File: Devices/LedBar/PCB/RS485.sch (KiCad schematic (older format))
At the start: 20 parts, among them J401 RS485, U401 ISO3082DW, U402 B0505S-1W-SIP4

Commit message: Renamed libraries
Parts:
- J401: footprint AmbientLight:15EDGRC-3.5-3P -> RGBW-Bar:15EDGRC-3.5-3P
- TP401, TP402, TP403, TP404, TP405, TP406, TP407, TP408, TP409: footprint AmbientLight:TestPoint_Pad_D1.0mm -> RGBW-Bar:TestPoint_Pad_D1.0mm
- U402: footprint AmbientLight:B0505S-1W -> RGBW-Bar:B0505S-1W; symbol AmbientLight:B0505S-1W-SIP4 -> RGBW-Bar:B0505S-1W-SIP4
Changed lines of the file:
@@
 F 0 "TP406" H 7658 4468 50  0000 L CNN
 F 1 "txd" H 7658 4377 50  0000 L CNN
-F 2 "AmbientLight:TestPoint_Pad_D1.0mm" H 7800 4350 50  0001 C CNN
+F 2 "RGBW-Bar:TestPoint_Pad_D1.0mm" H 7800 4350 50  0001 C CNN
 F 3 "~" H 7800 4350 50  0001 C CNN
 	1    7600 4350
@@
 F 0 "TP407" H 7542 4676 50  0000 R CNN
 F 1 "rxd" H 7542 4767 50  0000 R CNN
-F 2 "AmbientLight:TestPoint_Pad_D1.0mm" H 7800 4650 50  0001 C CNN
+F 2 "RGBW-Bar:TestPoint_Pad_D1.0mm" H 7800 4650 50  0001 C CNN
 F 3 "~" H 7800 4650 50  0001 C CNN
 	1    7600 4650
@@
 F 0 "TP408" H 7542 5076 50  0000 R CNN
 F 1 "tx_en" H 7542 5167 50  0000 R CNN
-F 2 "AmbientLight:TestPoint_Pad_D1.0mm" H 7800 5050 50  0001 C CNN
+F 2 "RGBW-Bar:TestPoint_Pad_D1.0mm" H 7800 5050 50  0001 C CNN
 F 3 "~" H 7800 5050 50  0001 C CNN
 	1    7600 5050
@@
 $EndComp
 $Comp
-L AmbientLight:GND_iso #PWR0407
+L RGBW-Bar:GND_iso #PWR0407
 U 1 1 6088C9C5
 P 6000 5300
@@
 $EndComp
 $Comp
-L AmbientLight:GND_iso #PWR0401
+L RGBW-Bar:GND_iso #PWR0401
 U 1 1 6088DF33
 P 3450 5300
@@
 	6000 5200 6000 5300
 $Comp
-L AmbientLight:GND_iso #PWR0402
+L RGBW-Bar:GND_iso #PWR0402
 U 1 1 60894182
 P 4600 5300
@@
 F 0 "J401" H 3150 4350 50  0000 C CNN
 F 1 "RS485" H 3450 4600 50  0000 R CNN
-F 2 "AmbientLight:15EDGRC-3.5-3P" H 3150 4600 50  0001 C CNN
+F 2 "RGBW-Bar:15EDGRC-3.5-3P" H 3150 4600 50  0001 C CNN
 F 3 "~" H 3150 4600 50  0001 C CNN
 	1    3150 4600
@@
 	4600 5150 4600 5300
 $Comp
-L AmbientLight:B0505S-1W-SIP4 U402
+L RGBW-Bar:B0505S-1W-SIP4 U402
 U 1 1 608B32EA
 P 6350 2250
 F 0 "U402" H 6350 2765 50  0000 C CNN
 F 1 "B0505S-1W-SIP4" H 6350 2674 50  0000 C CNN
-F 2 "AmbientLight:B0505S-1W" H 6100 2250 50  0001 C CNN
+F 2 "RGBW-Bar:B0505S-1W" H 6100 2250 50  0001 C CNN
 F 3 "https://datasheetspdf.com/pdf-file/792761/MORNSUN/B0505S-1W/1" H 6100 2250 50  0001 C CNN
 	1    6350 2250
@@
 Connection ~ 7100 2050
 $Comp
-L AmbientLight:GND_iso #PWR0405
+L RGBW-Bar:GND_iso #PWR0405
 U 1 1 608BCBD7
 P 5600 2550
@@
 $EndComp
 $Comp
-L AmbientLight:+5V_iso #PWR0404
+L RGBW-Bar:+5V_iso #PWR0404
 U 1 1 608BEF84
 P 5600 1950
@@
 	6000 3500 6000 3800
 $Comp
-L AmbientLight:+5V_iso #PWR0406
+L RGBW-Bar:+5V_iso #PWR0406
 U 1 1 6089173E
 P 5750 3350
@@
 	5750 3500 6000 3500
 $Comp
-L AmbientLight:GND_iso #PWR0403
+L RGBW-Bar:GND_iso #PWR0403
 U 1 1 608F11EC
 P 5500 3800
@@
 F 0 "TP404" H 5058 2118 50  0000 L CNN
 F 1 "+5V_iso" H 5058 2027 50  0000 L CNN
-F 2 "AmbientLight:TestPoint_Pad_D1.0mm" H 5200 2000 50  0001 C CNN
+F 2 "RGBW-Bar:TestPoint_Pad_D1.0mm" H 5200 2000 50  0001 C CNN
 F 3 "~" H 5200 2000 50  0001 C CNN
 	1    5000 2000
@@
 F 0 "TP405" H 4942 2526 50  0000 R CNN
 F 1 "GND_iso" H 4942 2617 50  0000 R CNN
-F 2 "AmbientLight:TestPoint_Pad_D1.0mm" H 5200 2500 50  0001 C CNN
+F 2 "RGBW-Bar:TestPoint_Pad_D1.0mm" H 5200 2500 50  0001 C CNN
 F 3 "~" H 5200 2500 50  0001 C CNN
 	1    5000 2500
@@
 F 0 "TP402" H 3658 4468 50  0000 L CNN
 F 1 "B" H 3658 4377 50  0000 L CNN
-F 2 "AmbientLight:TestPoint_Pad_D1.0mm" H 3800 4350 50  0001 C CNN
+F 2 "RGBW-Bar:TestPoint_Pad_D1.0mm" H 3800 4350 50  0001 C CNN
 F 3 "~" H 3800 4350 50  0001 C CNN
 	1    3600 4350
@@
 F 0 "TP403" H 3542 4676 50  0000 R CNN
 F 1 "A" H 3542 4767 50  0000 R CNN
-F 2 "AmbientLight:TestPoint_Pad_D1.0mm" H 3800 4650 50  0001 C CNN
+F 2 "RGBW-Bar:TestPoint_Pad_D1.0mm" H 3800 4650 50  0001 C CNN
 F 3 "~" H 3800 4650 50  0001 C CNN
 	1    3600 4650
@@
 F 0 "TP409" H 7542 5676 50  0000 R CNN
 F 1 "gnd" H 7542 5767 50  0000 R CNN
-F 2 "AmbientLight:TestPoint_Pad_D1.0mm" H 7800 5650 50  0001 C CNN
+F 2 "RGBW-Bar:TestPoint_Pad_D1.0mm" H 7800 5650 50  0001 C CNN
 F 3 "~" H 7800 5650 50  0001 C CNN
 	1    7600 5650
@@
 F 0 "TP401" V 3550 5150 50  0000 C CNN
 F 1 "GND_iso" V 3392 5117 50  0000 C CNN
-F 2 "AmbientLight:TestPoint_Pad_D1.0mm" H 3650 5000 50  0001 C CNN
+F 2 "RGBW-Bar:TestPoint_Pad_D1.0mm" H 3650 5000 50  0001 C CNN
 F 3 "~" H 3650 5000 50  0001 C CNN
 	1    3450 5000

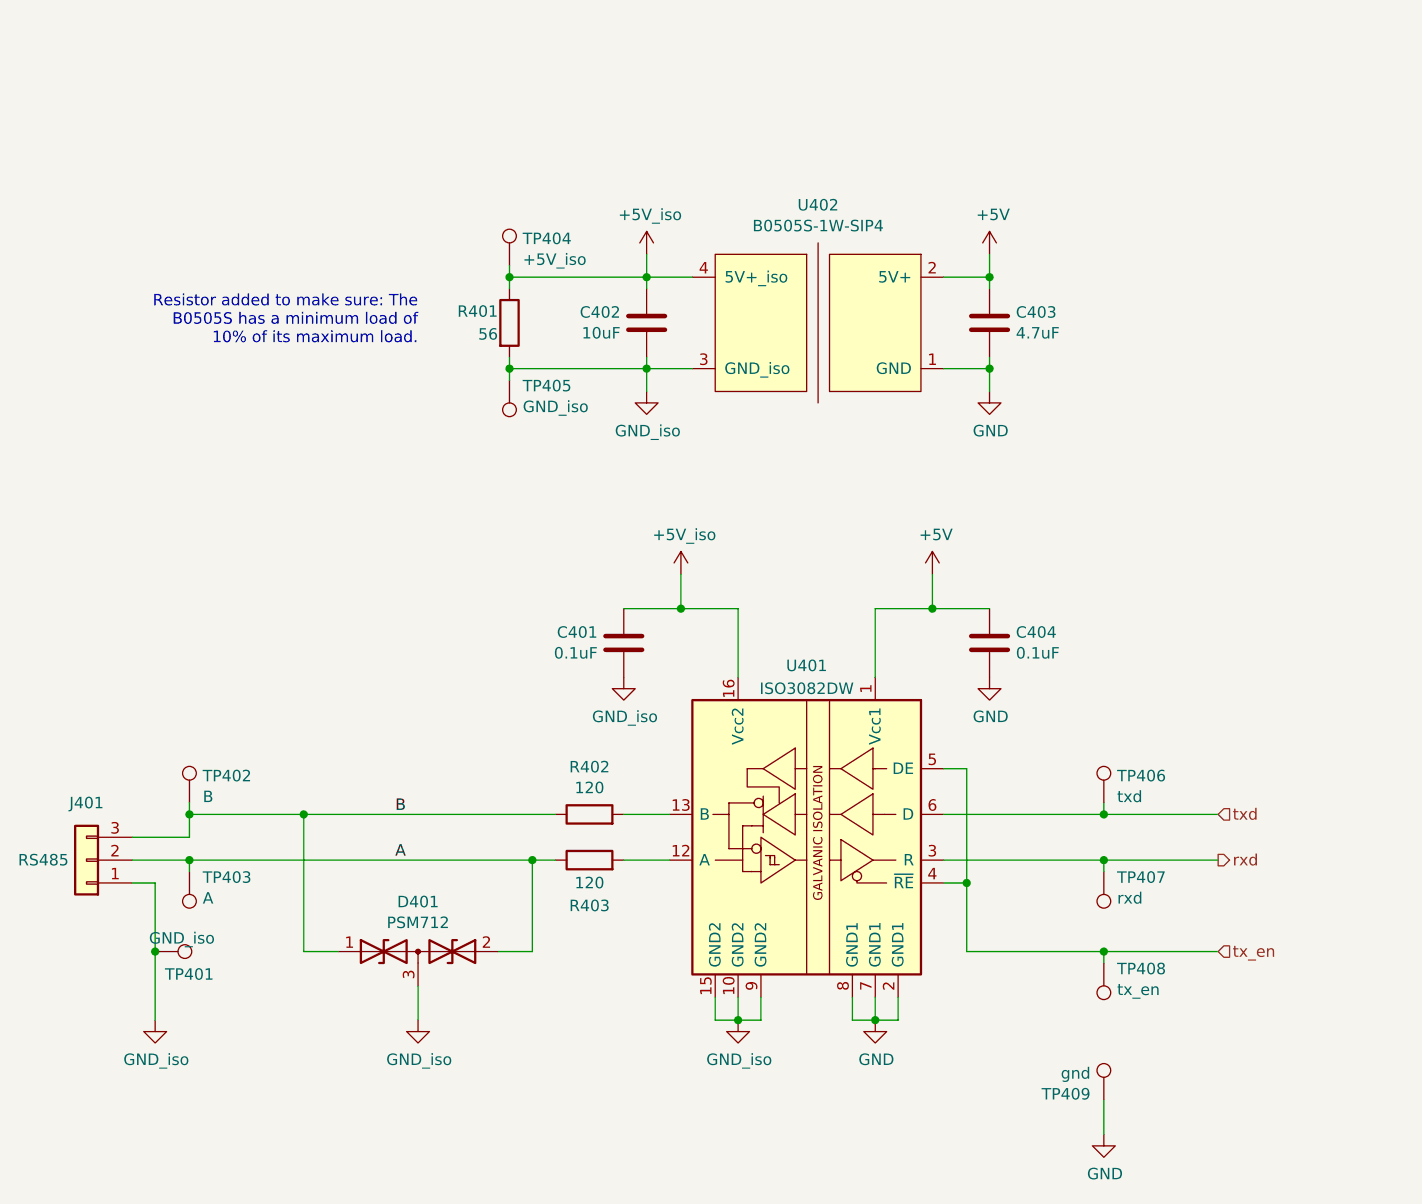
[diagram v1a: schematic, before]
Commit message: Cosmetic changes to shematics
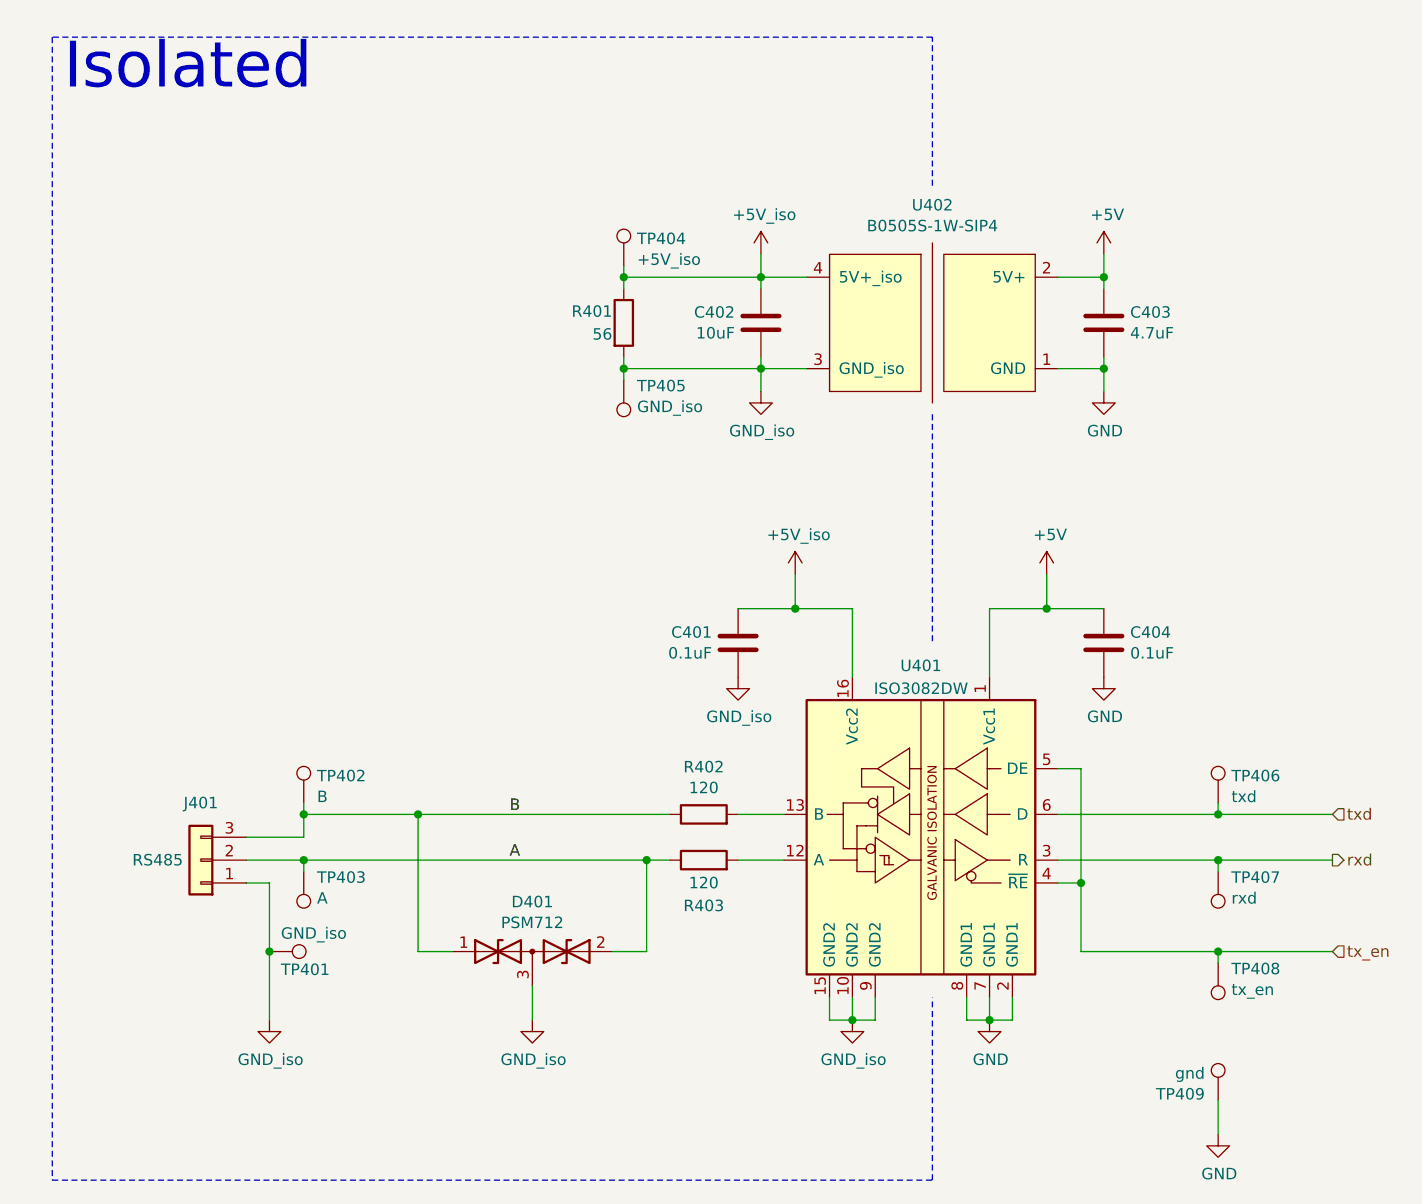
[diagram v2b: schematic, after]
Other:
- note added: "Isolated"
- note removed: "Resistor added to make sure: The\nB0505S has a minimum load of\n10% of its maximum load."
- moved on the sheet: C401, C402, C403, C404, D401, J401, R401, R402, R403, TP401, TP402, TP403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
